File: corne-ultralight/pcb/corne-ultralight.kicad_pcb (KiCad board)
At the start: 2 copper layers, 275.5 x 105.6 mm, 148 parts, among them J2 OLED, J5 Breakaway_Tabs, J7 OLED, SW1 SW_PUSH, SW10 SW_PUSH, SW11 SW_PUSH, SW12 SW_PUSH, SW13 SW_PUSH, SW14 SW_PUSH, SW15 SW_PUSH, SW16 SW_PUSH, SW17 SW_PUSH, SW18 SW_PUSH, SW19 SW_PUSH, SW2 SW_PUSH, SW20 SW_PUSH, SW21 SW_PUSH, SW22 SW_PUSH, SW23 SW_PUSH, SW24 SW_PUSH, SW25 SW_PUSH, SW26 SW_PUSH, SW27 SW_PUSH, SW28 SW_PUSH, SW29 SW_PUSH, SW3 SW_PUSH, SW30 SW_PUSH, SW31 SW_PUSH, SW32 SW_PUSH, SW33 SW_PUSH, SW34 SW_PUSH, SW35 SW_PUSH, SW36 SW_PUSH, SW37 SW_PUSH, SW38 SW_PUSH, SW39 SW_PUSH, SW4 SW_PUSH, SW40 SW_PUSH, SW41 SW_PUSH, SW42 SW_PUSH, SW5 SW_PUSH, SW6 SW_PUSH, SW7 SW_PUSH, SW8 SW_PUSH, SW9 SW_PUSH, U1 ProMicro, U2 ProMicro

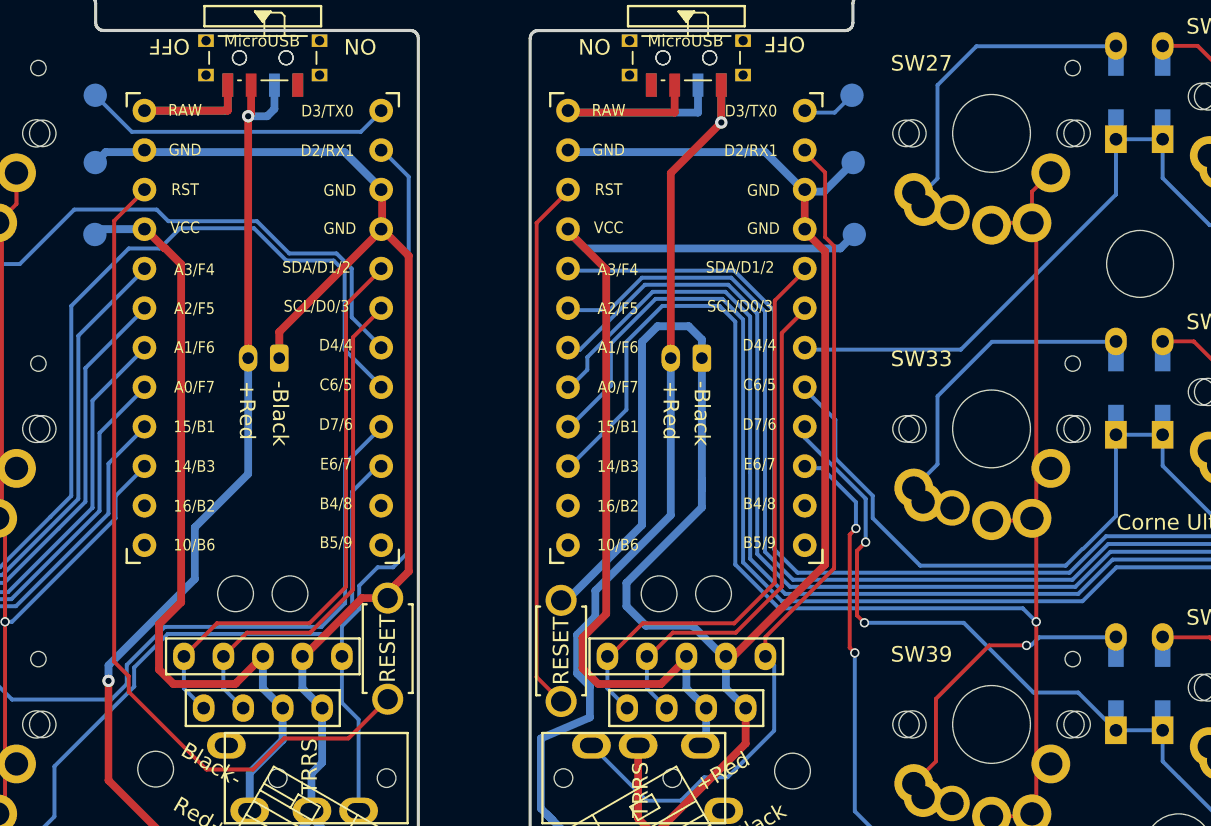
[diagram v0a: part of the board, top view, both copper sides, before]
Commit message: Updates
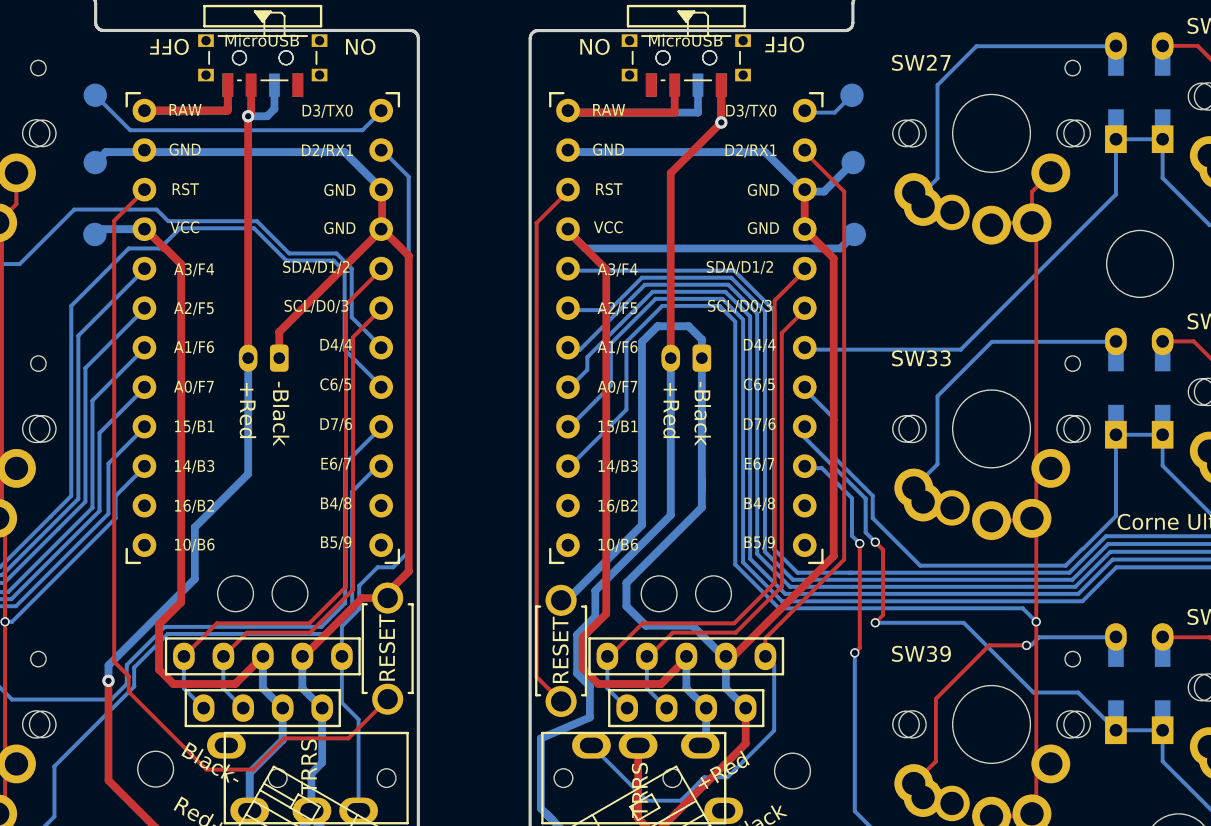
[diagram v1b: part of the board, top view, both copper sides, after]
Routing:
- net CS_r: track 55.3 -> 55.8 mm
